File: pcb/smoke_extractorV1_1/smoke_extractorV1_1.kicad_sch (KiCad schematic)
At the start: 36 parts

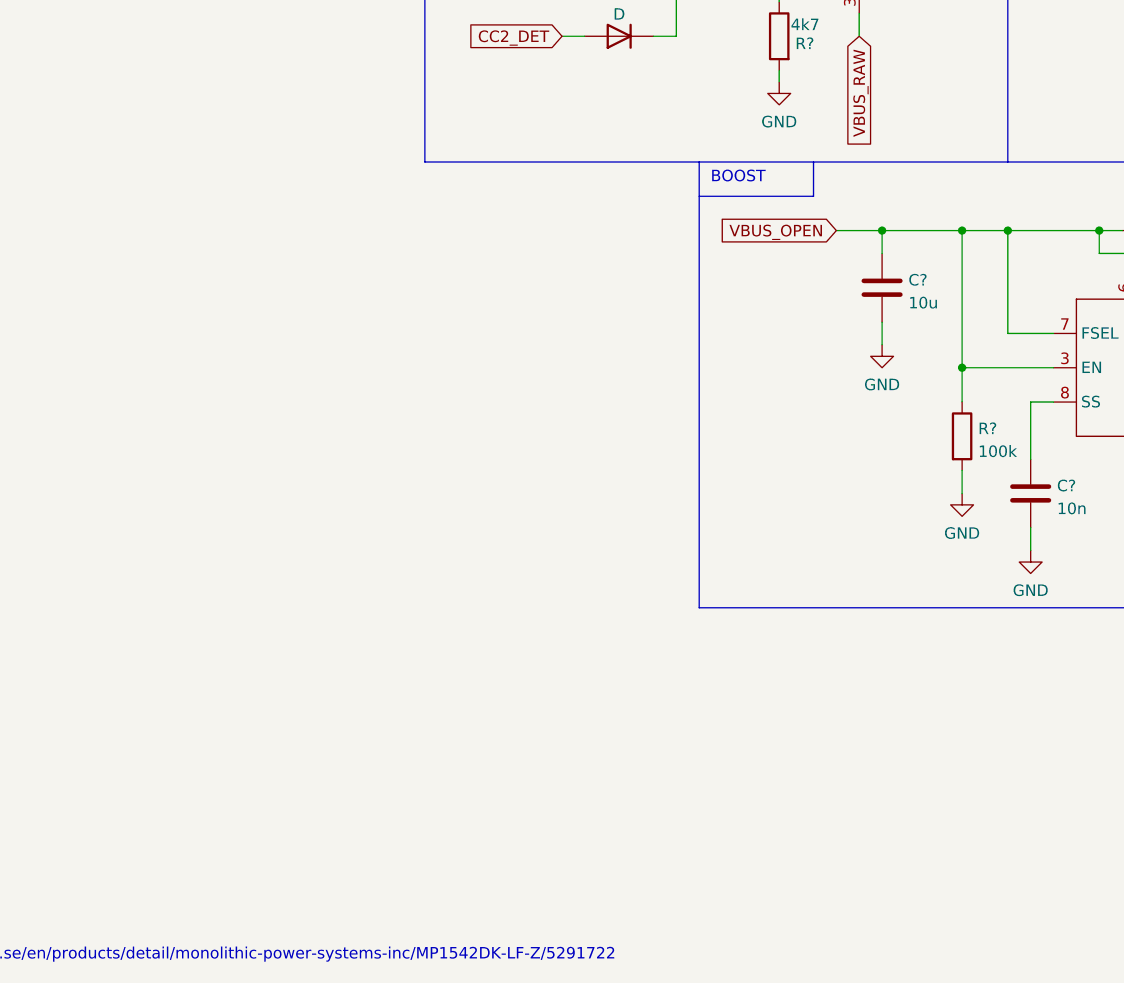
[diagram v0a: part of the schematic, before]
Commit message: Final schematics tweaks and BOM
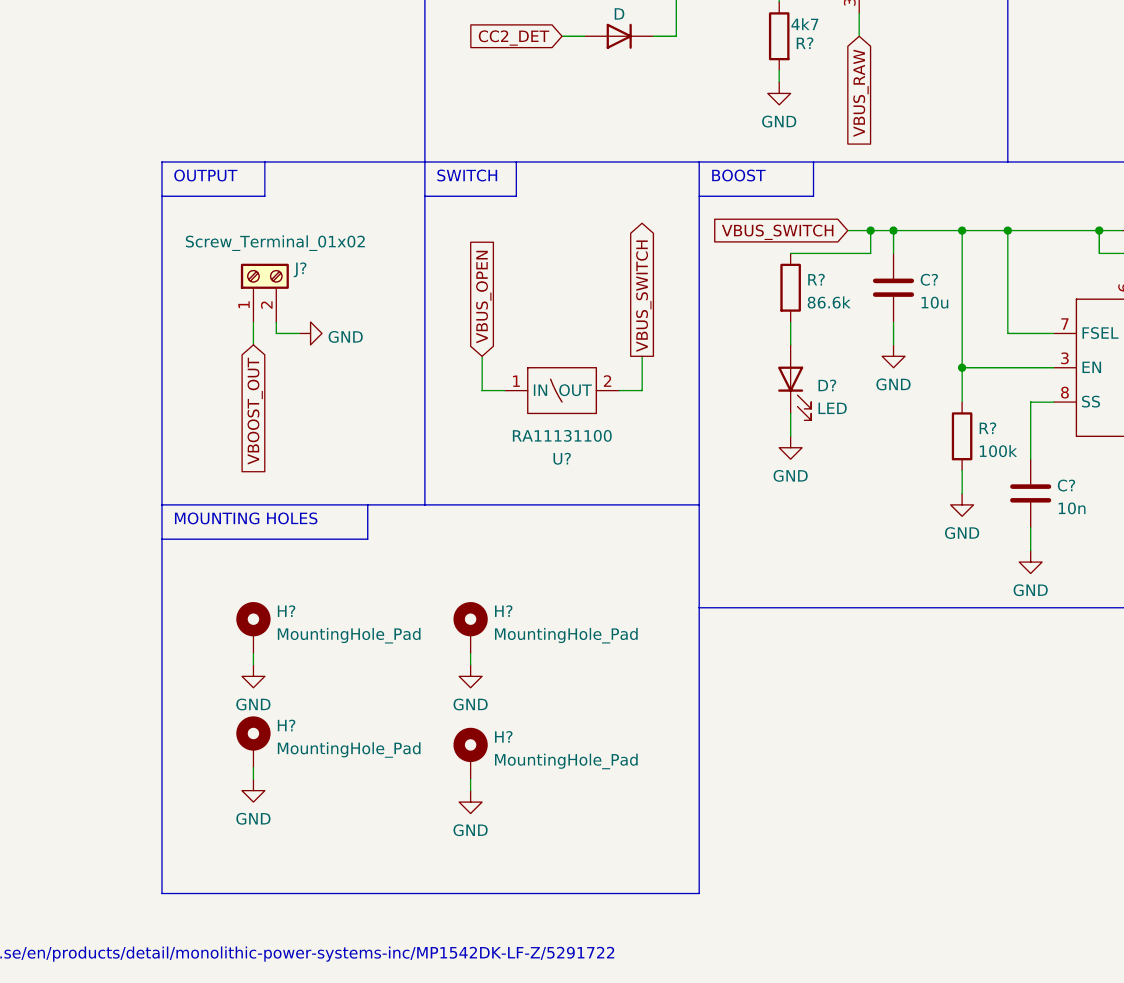
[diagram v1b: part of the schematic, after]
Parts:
- added D?: LED, symbol Device:LED
- added H? (x4): MountingHole_Pad, symbol Mechanical:MountingHole_Pad
- added J?: Screw_Terminal_01x02, symbol Connector:Screw_Terminal_01x02
- added R?: 86.6k, symbol Device:R
- added U?: RA11131100, symbol CustomSymbols:RA11131100
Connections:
- net GND: now also D?.1 (K), H?.1, H?.1, H?.1, H?.1, J?.2 (Pin_2)
- net VBOOST_OUT: now also J?.1 (Pin_1)
- net VBUS_OPEN: now also U?.1 (IN); no longer C?.1, L?.1, R?.1, U?.3 (EN), U?.6 (IN), U?.7 (FSEL)
- new net: D?.2 (A), R?.2
- new net VBUS_SWITCH: C?.1, L?.1, R?.1, R?.1, U?.2 (OUT), U?.3 (EN), U?.6 (IN), U?.7 (FSEL)
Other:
- note added: "MOUNTING HOLES"
- note added: "OUTPUT"
- note added: "SWITCH"
- moved on the sheet: C?
